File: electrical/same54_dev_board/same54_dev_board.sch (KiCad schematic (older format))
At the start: 0 parts

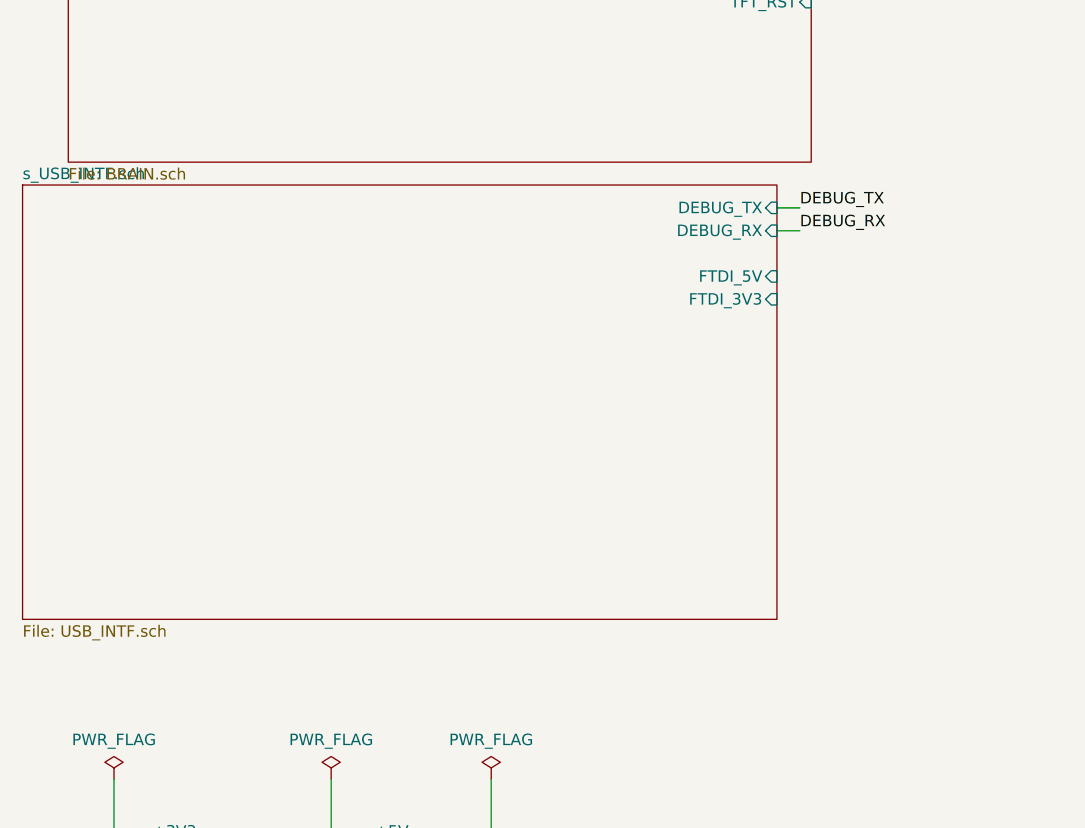
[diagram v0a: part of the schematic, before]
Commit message: migrating to laptop
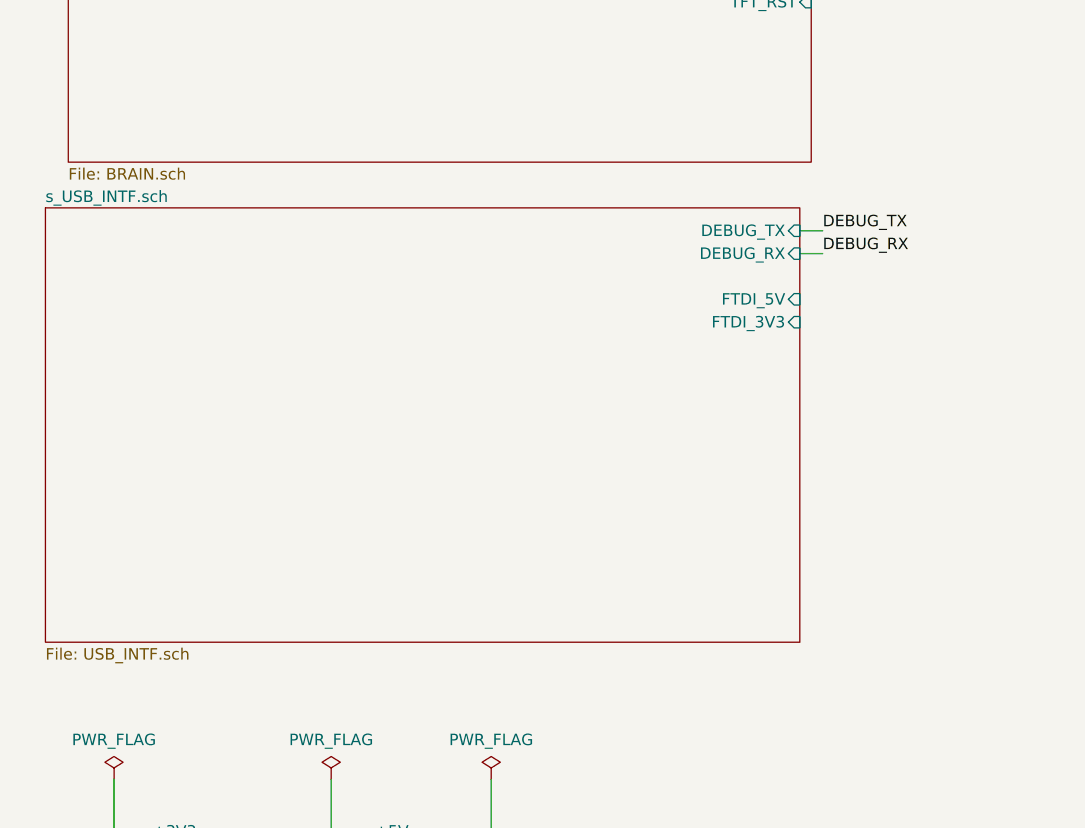
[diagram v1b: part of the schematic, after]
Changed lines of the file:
@@
 	5750 2300 5700 2300
 Wire Wire Line
-	3850 3450 3950 3450
+	3950 3550 4050 3550
 Wire Wire Line
-	3850 3350 3950 3350
-Text Label 3950 3450 0    50   ~ 0
+	3950 3450 4050 3450
+Text Label 4050 3550 0    50   ~ 0
 DEBUG_RX
-Text Label 3950 3350 0    50   ~ 0
+Text Label 4050 3450 0    50   ~ 0
 DEBUG_TX
 $Sheet
-S 550  3250 3300 1900
+S 650  3350 3300 1900
 U 5E7C0F59
 F0 "s_USB_INTF.sch" 50
 F1 "USB_INTF.sch" 50
-F2 "DEBUG_TX" I R 3850 3350 50
-F3 "DEBUG_RX" I R 3850 3450 50
-F4 "FTDI_5V" I R 3850 3650 50
-F5 "FTDI_3V3" I R 3850 3750 50
+F2 "DEBUG_TX" I R 3950 3450 50
+F3 "DEBUG_RX" I R 3950 3550 50
+F4 "FTDI_5V" I R 3950 3750 50
+F5 "FTDI_3V3" I R 3950 3850 50
 $EndSheet
 $Sheet
